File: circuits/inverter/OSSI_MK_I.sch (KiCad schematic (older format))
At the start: 0 parts

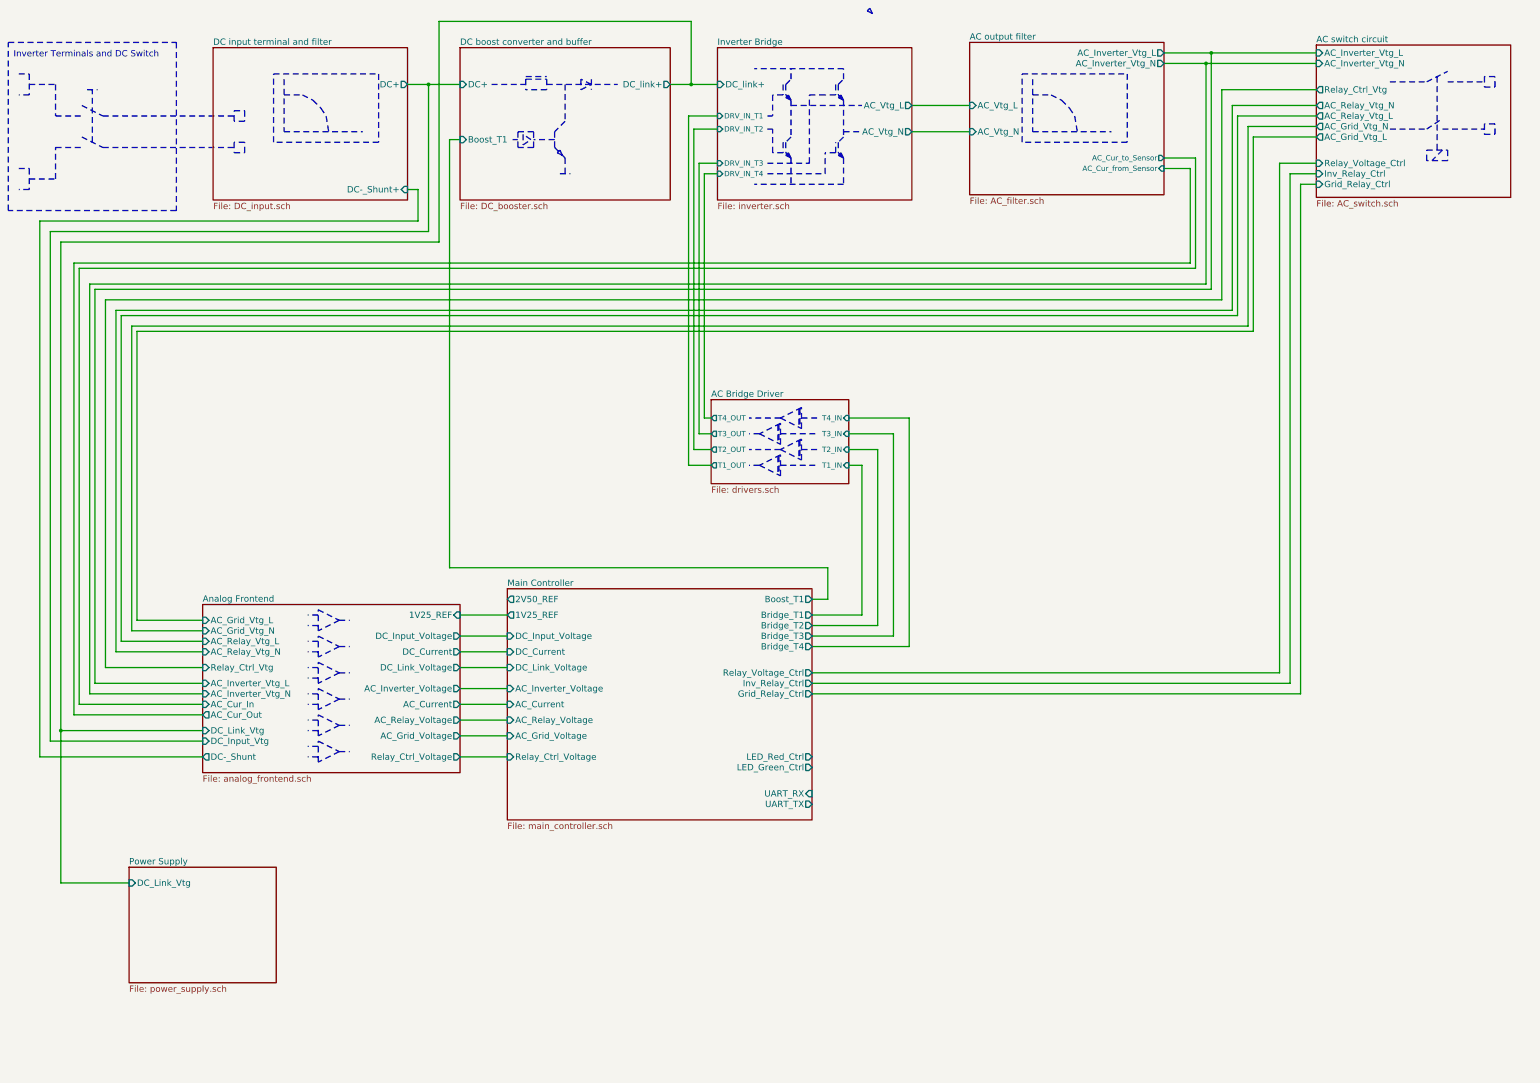
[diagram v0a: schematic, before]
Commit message: minor updates and cleaup
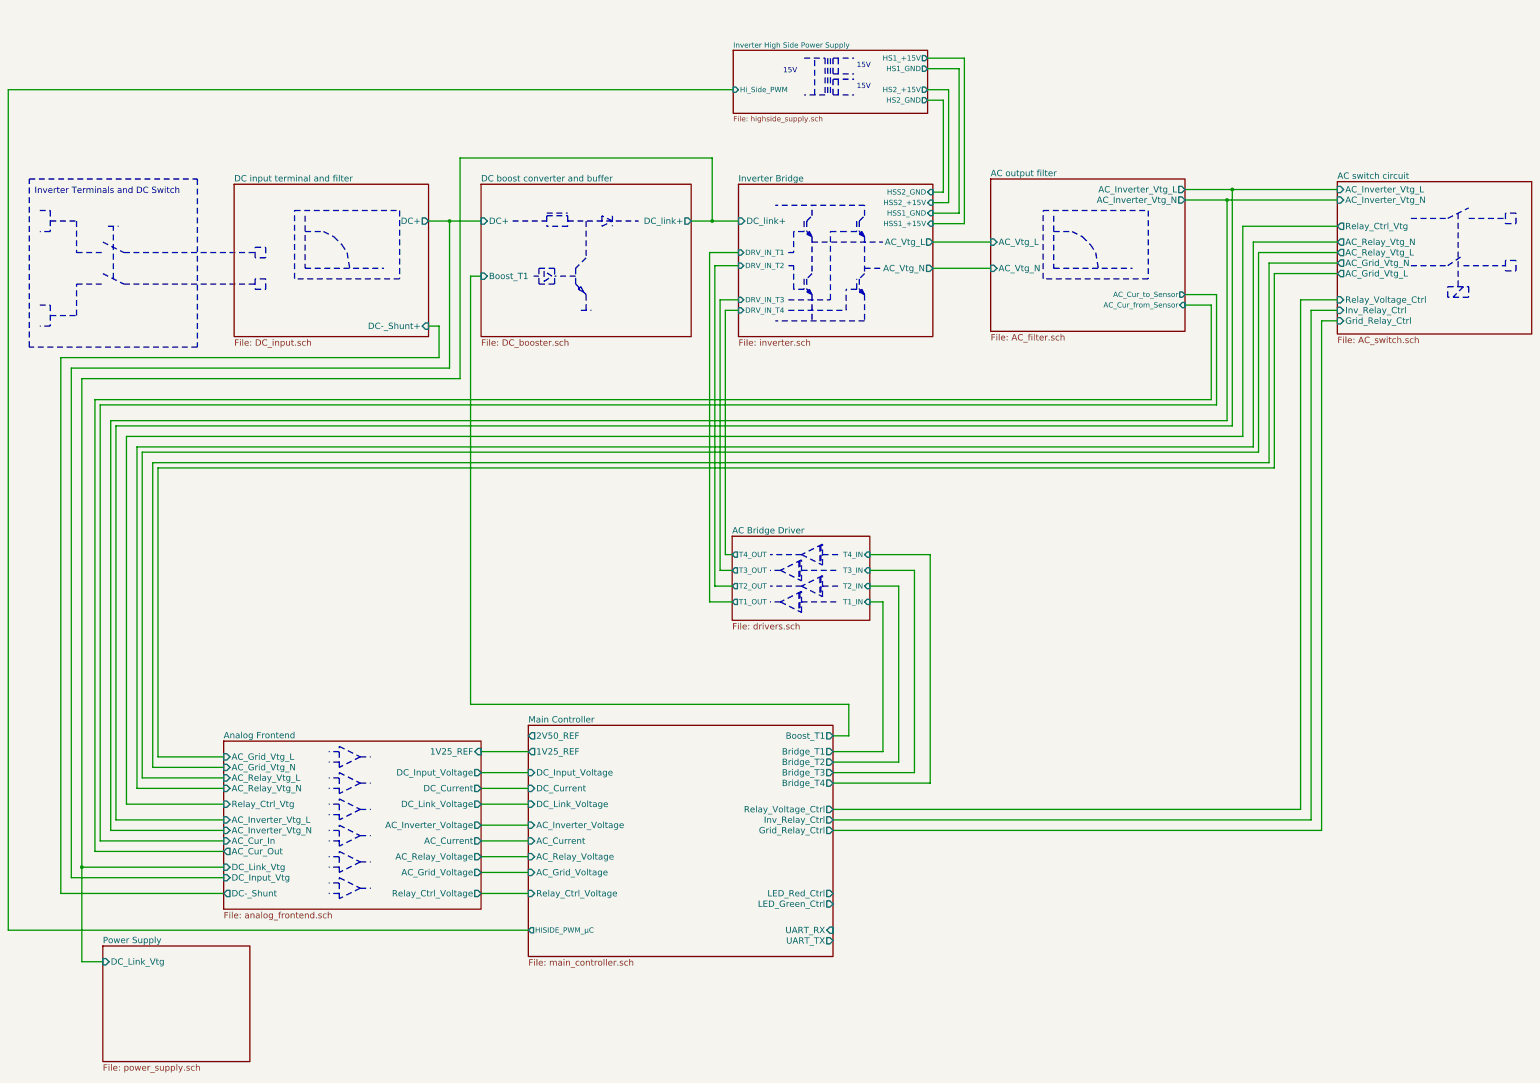
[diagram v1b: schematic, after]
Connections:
- wire segments 117 -> 132
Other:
- note added: "15V"
- note added: "15V\n"
